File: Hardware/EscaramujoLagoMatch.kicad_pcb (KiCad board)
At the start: 2 copper layers, 113 x 80 mm, 32 parts, among them J1 TP_3v3, J10 I2C, J2 RJ45, J3 TP_5V, J4 TP_GND, J5 TEMP_PRES, J6 TP_12V, J7 RedPitaya, J8 TP_PMT_CTL_V, J9 TP_GND, U1 MAX662A, U2 MAX604, U3 MAX603, U4 MCP41100, U5 LM358

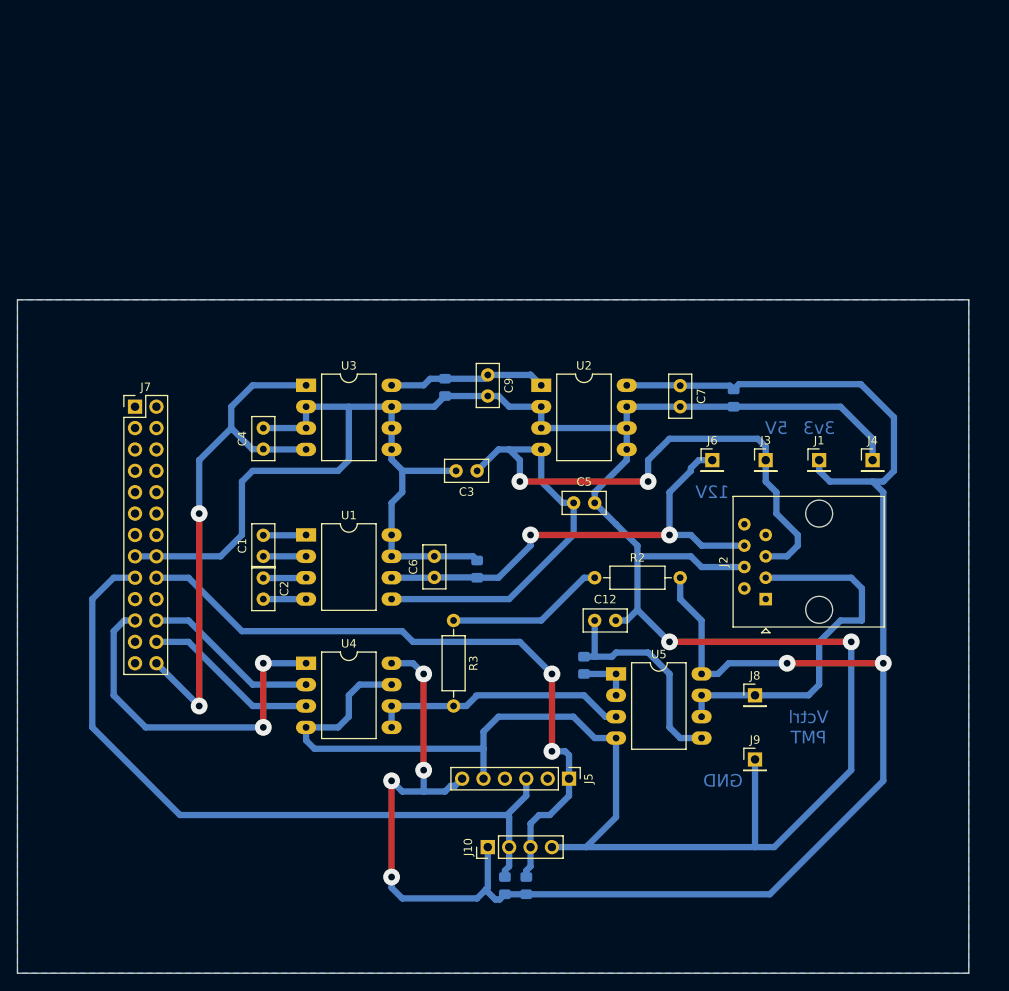
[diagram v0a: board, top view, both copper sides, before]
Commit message: Add files via upload
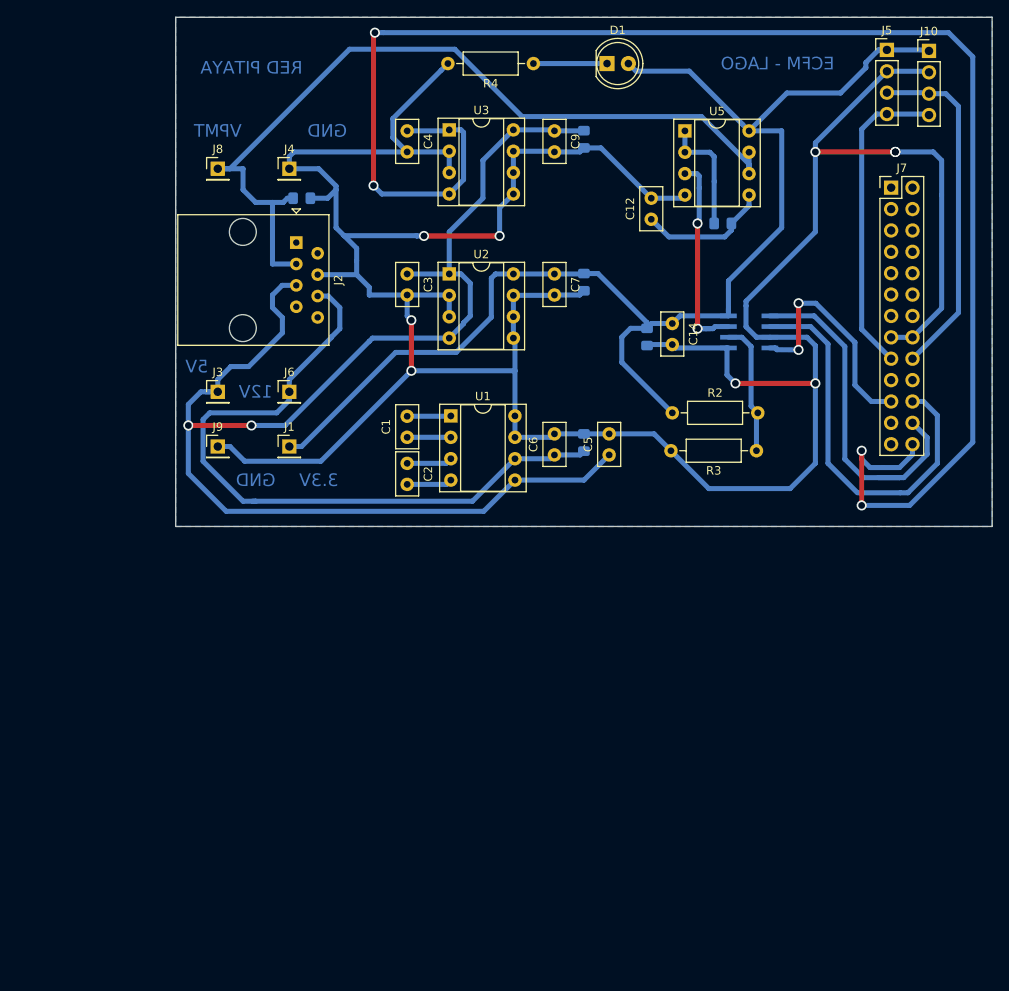
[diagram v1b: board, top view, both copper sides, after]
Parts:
- removed R5: 4k7, Resistor_SMD:R_0805_2012Metric_Pad1.15x1.40mm_HandSolder
- added C13: 100n, Capacitor_SMD:C_0805_2012Metric_Pad1.15x1.40mm_HandSolder, B.Cu at (87.5, 120.0)
- added C14: 10u, Capacitor_THT:C_Disc_D5.0mm_W2.5mm_P2.50mm, F.Cu at (90.5, 118.4)
- added C15: 100n, Capacitor_SMD:C_0805_2012Metric_Pad1.15x1.40mm_HandSolder, B.Cu at (46.5, 103.5)
- added D1: LED, LED_THT:LED_D5.0mm, F.Cu at (82.7, 87.5)
- J5: value TEMP_PRES -> Sensor; footprint Connector_PinHeader_2.54mm:PinHeader_1x06_P2.54mm_Vertical -> Connector_PinHeader_2.54mm:PinHeader_1x04_P2.54mm_Vertical
- R2: value 15k -> 5.1k
- R3: value 18k -> 3k
- R4: value 4k7 -> 330; footprint Resistor_SMD:R_0805_2012Metric_Pad1.15x1.40mm_HandSolder -> Resistor_THT:R_Axial_DIN0207_L6.3mm_D2.5mm_P10.16mm_Horizontal; moved to F.Cu
- U1, U2, U3, U5: footprint Package_DIP:DIP-8_W10.16mm_LongPads -> Package_DIP:DIP-8_W7.62mm_Socket
- U4: value MCP41100 -> TLV5616CD; footprint Package_DIP:DIP-8_W10.16mm_LongPads -> SOIC127P600X175-8N; moved to B.Cu
- moved J10 108.1 mm to (121.0, 86.0), turned to 0 degrees
- moved R4 97.7 mm to (74.0, 87.5), turned to 180 degrees
- moved J5 94.5 mm to (116.0, 85.9), turned to 0 degrees
- moved J7 93.5 mm to (116.5, 102.2)
- moved J8 89.4 mm to (36.5, 100.0)
- moved J4 77.5 mm to (45.0, 100.0)
- moved J9 73.9 mm to (36.5, 133.0)
- moved J2 70.0 mm to (45.8, 108.8), turned to 270 degrees
- moved U4 65.7 mm to (99.6, 119.4), turned to 180 degrees
- moved J3 65.6 mm to (36.5, 126.5)
- moved U5 65.0 mm to (92.0, 95.5)
- moved J1 63.0 mm to (45.0, 133.0)
- moved R1 55.0 mm to (96.5, 106.5), turned to 180 degrees
- moved J6 50.9 mm to (45.0, 126.5)
- moved C12 48.1 mm to (88.0, 106.0), turned to 90 degrees
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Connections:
- J10 pad 2: /I2C_SDA -> GND
- J10 pad 4: GND -> /I2C_SDA
- J2 pad 1: (no net) -> Net-(J2-Pad1)
- J2 pad 2: (no net) -> Net-(J2-Pad2)
- J2 pad 7: (no net) -> Net-(J2-Pad7)
- J2 pad 8: (no net) -> Net-(J2-Pad8)
- J5 pad 1: /I2C_SCL -> +3V3
- J5 pad 2: (no net) -> GND
- J5 pad 3: /I2C_SDA -> /I2C_SCL
- J5 pad 4: (no net) -> /I2C_SDA
- J7 pad 1: (no net) -> Net-(J7-Pad1)
- J7 pad 10: (no net) -> Net-(J7-Pad10)
- J7 pad 11: (no net) -> Net-(J7-Pad11)
- J7 pad 12: (no net) -> Net-(J7-Pad12)
- J7 pad 13: (no net) -> Net-(J7-Pad13)
- J7 pad 14: (no net) -> Net-(J7-Pad14)
- J7 pad 19: (no net) -> Net-(J7-Pad19)
- J7 pad 2: (no net) -> Net-(J7-Pad2)
- J7 pad 20: (no net) -> Net-(J7-Pad20)
- J7 pad 23: (no net) -> Net-(J7-Pad23)
- J7 pad 25: (no net) -> Net-(J7-Pad25)
- J7 pad 3: (no net) -> Net-(J7-Pad3)
- J7 pad 4: (no net) -> Net-(J7-Pad4)
- J7 pad 5: (no net) -> Net-(J7-Pad5)
- J7 pad 6: (no net) -> Net-(J7-Pad6)
- J7 pad 7: (no net) -> Net-(J7-Pad7)
- J7 pad 8: (no net) -> Net-(J7-Pad8)
- J7 pad 9: (no net) -> Net-(J7-Pad9)
- R2 pad 1: Net-(R2-Pad1) -> +3V3
- R2 pad 2: +3V3 -> Net-(R2-Pad2)
- R3 pad 1: Net-(R2-Pad1) -> Net-(R2-Pad2)
- R3 pad 2: Net-(R3-Pad2) -> GND
- R4 pad 1: +3V3 -> Net-(D1-Pad1)
- R4 pad 2: /I2C_SCL -> GND
- U4 pad 1: /SPI_CS -> /SPI_MOSI
- U4 pad 3: /SPI_MOSI -> GND
- U4 pad 4: GND -> /SPI_CS
- U4 pad 5: Net-(R3-Pad2) -> GND
- U4 pad 6: Net-(R3-Pad2) -> Net-(R2-Pad2)
- U4 pad 7: GND -> Net-(U4-Pad7)
- U5 pad 3: Net-(R3-Pad2) -> Net-(U4-Pad7)
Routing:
- net /5V_UNREG: track 64.2 -> 192.7 mm, vias 2 -> 4
- net +3V3: track 233.9 -> 154.3 mm, vias 6 -> 0
- net /PMT_CTRL_V: track 44.0 -> 100.7 mm
- net /I2C_SDA: track 88.3 -> 38.0 mm
- net +5V: track 120.0 -> 167.9 mm
- net /I2C_SCL: track 80.5 -> 41.4 mm, vias 2 -> 0
- net Net-(R3-Pad2): track 30.7 -> 0.00 mm
- net /SPI_CLK: track 20.9 -> 47.0 mm
- net /12V: track 57.2 -> 82.9 mm, vias 2 -> 0
- net Net-(U4-Pad7): track 0.00 -> 24.5 mm, vias 0 -> 2
- net /SPI_MOSI: track 20.9 -> 42.6 mm
- net Net-(R2-Pad1): track 18.9 -> 0.00 mm
- net Net-(R2-Pad2): track 0.00 -> 15.9 mm
- net /SPI_CS: track 42.7 -> 27.9 mm
- net Net-(C12-Pad1): track 26.4 -> 15.8 mm
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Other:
- board size 113 x 80 mm -> 97 x 60.5 mm
- net class Default: clearance 0.2 -> 0.6; trace_width 0.75 -> 0.6; via_dia 2 -> 1.2
- rule pad_to_mask_clearance: 0.2 -> 0
- rule trace_clearance: 0.2 -> 0.6
- rule trace_min: 0.4 -> 0.2
- rule via_min_drill: 0.4 -> 0.3
- rule via_min_size: 0.8 -> 0.4
- board text added: "3.3V"
- board text added: "ECFM - LAGO"
- board text added: "RED PITAYA"
- board text added: "VPMT"
- board text removed: "3v3"
- board text removed: "Vctrl PMT"
